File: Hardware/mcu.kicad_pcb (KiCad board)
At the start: 4 copper layers, 44 parts, among them T1 SCT-013-000, U1 INA128, U2 MCP6002-xMS, U3 ADS8688, U4 STM32F401CCUx

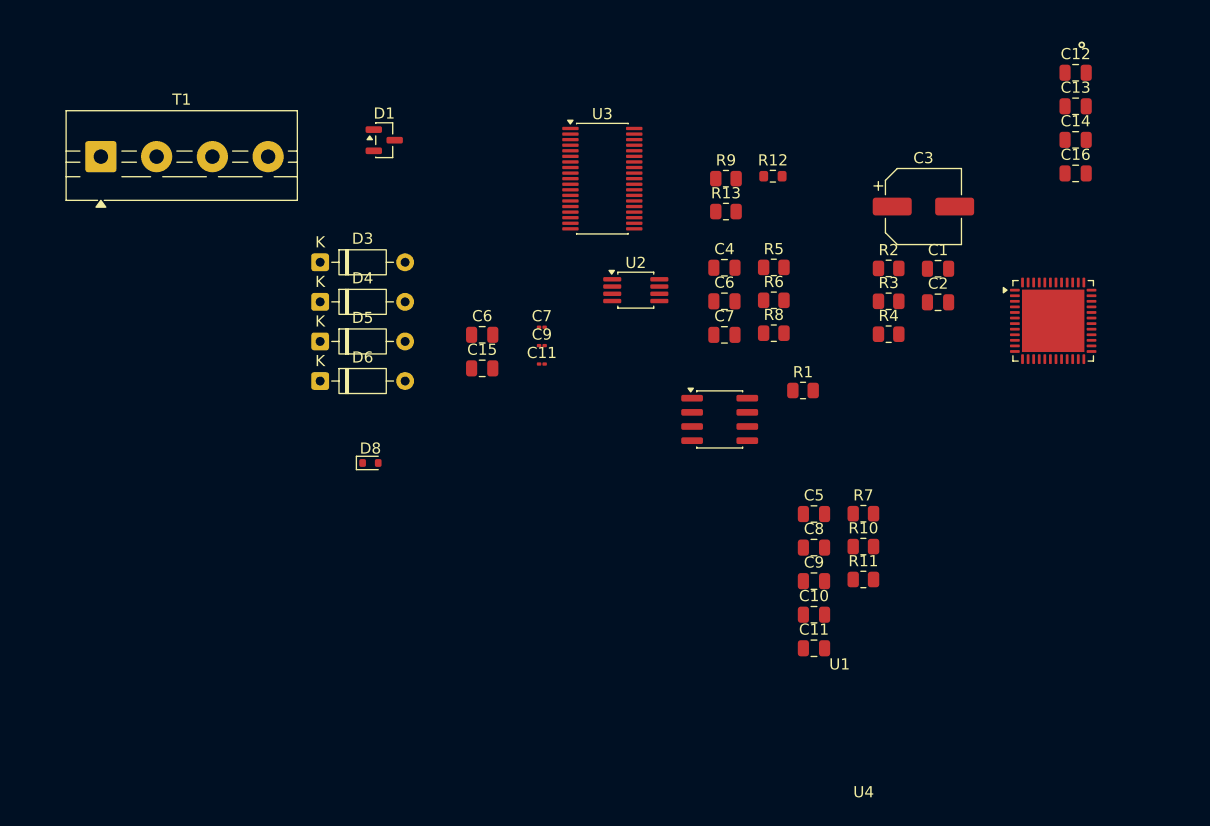
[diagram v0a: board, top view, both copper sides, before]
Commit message: completed hardware
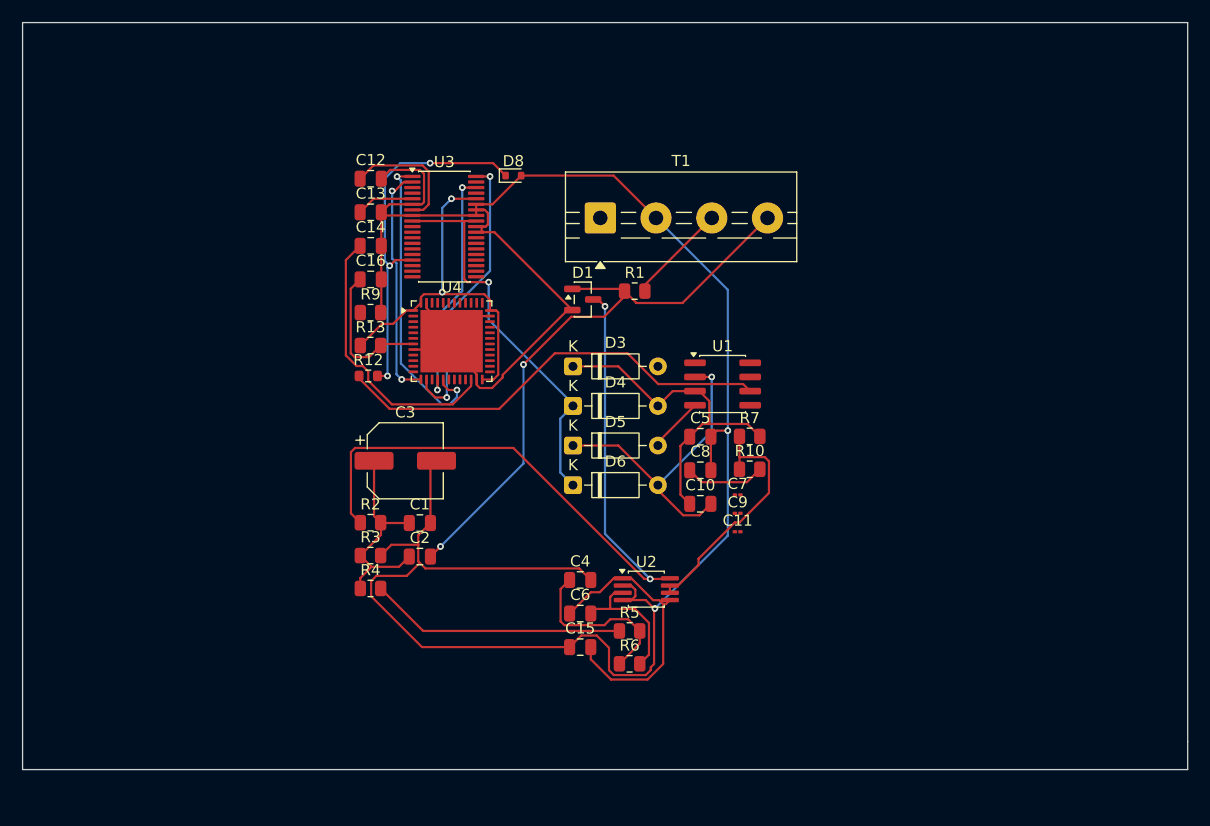
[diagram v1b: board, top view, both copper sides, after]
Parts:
- removed the C11 at (143.0, 124.6)
- removed the C11 at (118.6, 99.1)
- removed the C6 at (134.9, 93.5)
- removed the C6 at (113.2, 96.5)
- removed the C7 at (134.9, 96.5)
- removed the C7 at (118.6, 95.8)
- removed the C9 at (143.0, 118.6)
- removed the C9 at (118.6, 97.5)
- removed R11: R, Resistor_SMD:R_0805_2012Metric
- removed R8: 10k, Resistor_SMD:R_0805_2012Metric
- added C11: 100n, Capacitor_SMD:C_01005_0402Metric, F.Cu at (136.1, 114.2)
- added C6: 510p, Capacitor_SMD:C_0805_2012Metric, F.Cu at (122.0, 121.5)
- added C7: 100n, Capacitor_SMD:C_01005_0402Metric, F.Cu at (136.1, 110.9)
- added C9: 100n, Capacitor_SMD:C_01005_0402Metric, F.Cu at (136.1, 112.5)
- moved C12 63.9 mm to (103.2, 82.5)
- moved C13 63.9 mm to (103.2, 85.5)
- moved C14 63.9 mm to (103.2, 88.5)
- moved C16 63.9 mm to (103.2, 91.5)
- moved U4 54.0 mm to (110.5, 97.1)
- moved C1 51.8 mm to (107.6, 113.4)
- moved C3 51.8 mm to (106.3, 107.8)
- moved R2 51.8 mm to (103.2, 113.4)
- moved R3 51.8 mm to (103.2, 116.3)
- moved C2 51.8 mm to (107.6, 116.4)
- moved R4 51.8 mm to (103.2, 119.3)
- moved T1 45.1 mm to (123.8, 86.0)
- moved R12 40.5 mm to (103.0, 100.2)
- moved R5 35.1 mm to (126.4, 123.1)
- moved R6 35.1 mm to (126.4, 126.0)
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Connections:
- net /anti_aliasing/Out renamed /instrumentation_amplifier/INA128_input
- net /instrumentation_amplifier/Out renamed /instrumentation_amplifier/INA128_Output
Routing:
- net GND: track 0.00 -> 215.5 mm, vias 0 -> 2
- net VCC: track 0.00 -> 67.8 mm, vias 0 -> 2
- net /DC_Bias/In: track 0.00 -> 53.9 mm, vias 0 -> 2
- net /instrumentation_amplifier/INA128_Output: track 0.00 -> 39.9 mm
- net +5V: track 0.00 -> 35.5 mm, vias 0 -> 1
- net +3.3V: track 0.00 -> 34.1 mm, vias 0 -> 2
- net Net-(D8-K): track 0.00 -> 33.0 mm, vias 0 -> 3
- net Net-(D3-K): track 0.00 -> 30.6 mm
- net Net-(D5-K): track 0.00 -> 28.8 mm, vias 0 -> 1
- net Net-(U3-SDI): track 0.00 -> 27.6 mm, vias 0 -> 2
- net Net-(U2B-+): track 0.00 -> 25.7 mm
- net Net-(U3-~{CS}): track 0.00 -> 25.6 mm, vias 0 -> 2
- net Net-(U4-VCAP1): track 0.00 -> 25.2 mm
- net /DC_Bias/Out: track 0.00 -> 23.0 mm
- net /instrumentation_amplifier/INA128_input: track 0.00 -> 21.9 mm
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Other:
- board outline added: 104.5 x 67 mm
